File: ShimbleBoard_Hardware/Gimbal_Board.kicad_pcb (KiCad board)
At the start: 2 copper layers, 85 parts, among them Q1 Q_NMOS_GDS, Q2 Q_NMOS_GDS, Q3 Q_NMOS_GDS, Q4 Q_NMOS_GDS, Q5 Q_NMOS_GDS, Q6 Q_NMOS_GDS, Q7 Q_NMOS_GDS, Q8 Q_NMOS_GDS, SW1 SW_Push, SW10 SW_SPDT, SW2 SW_Push, SW3 SW_Push, SW4 SW_Push, SW5 SW_Push, SW6 SW_Push, SW7 SW_Push, SW8 SW_Push, SW9 SW_Push, U1 TM4C129E_Launchpad, U2 OKI, U3 OKI

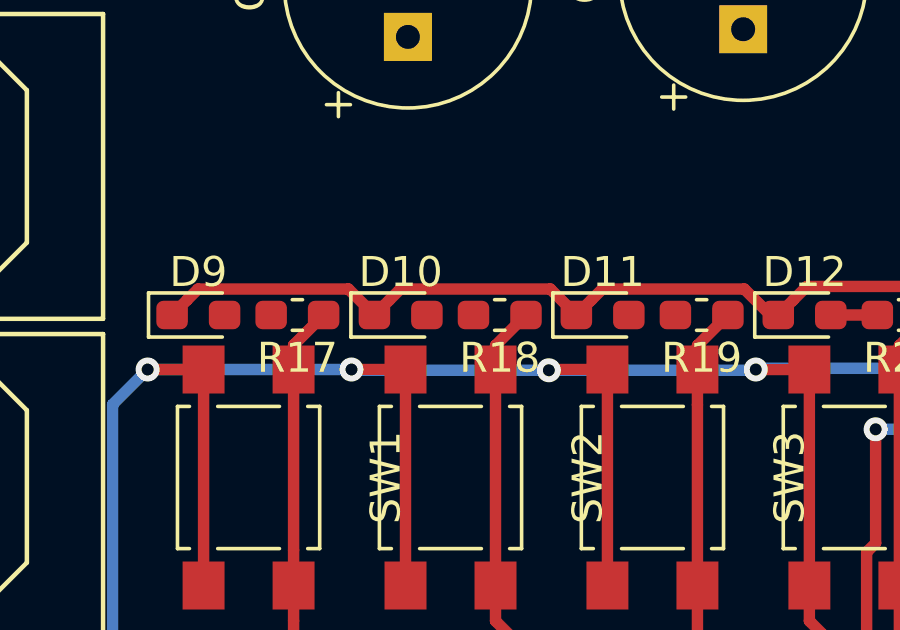
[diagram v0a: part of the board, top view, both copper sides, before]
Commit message: All Connected I Believe
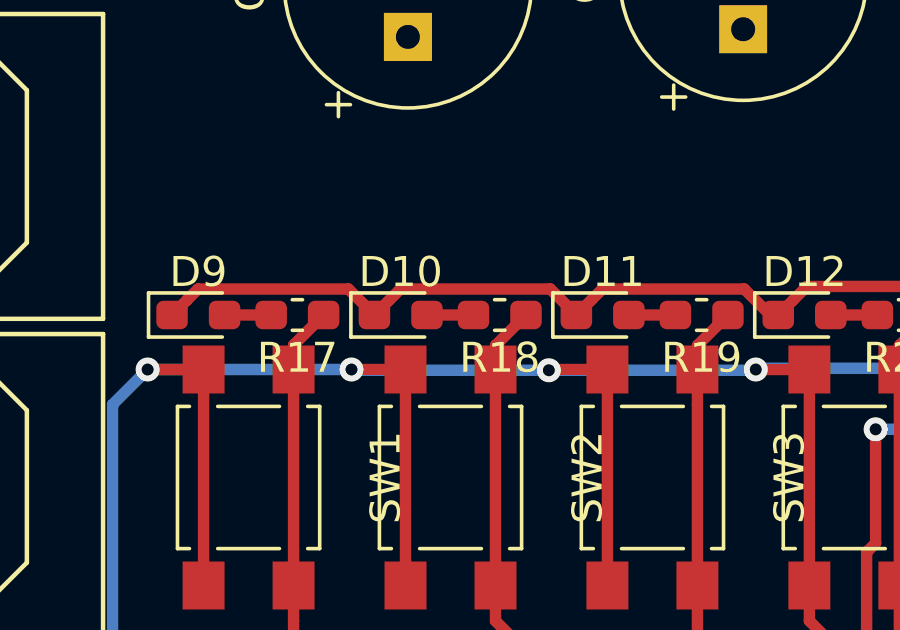
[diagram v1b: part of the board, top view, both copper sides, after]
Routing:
- net Net-(D9-Pad2): track 0.00 -> 1.55 mm
- net Net-(D11-Pad2): track 0.00 -> 1.55 mm
- net Net-(D10-Pad2): track 0.00 -> 1.55 mm
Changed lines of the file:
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@@
     (thickness 1.6)
     (drawings 1)
-    (tracks 401)
+    (tracks 404)
     (zones 0)
     (modules 85)
@@
   (segment (start 162.052 66.576) (end 162.842 65.786) (width 0.381) (layer F.Cu) (net 29))
   (segment (start 162.052 67.31) (end 162.052 66.576) (width 0.381) (layer F.Cu) (net 29))
+  (segment (start 113.27 90.551) (end 114.822 90.551) (width 0.381) (layer F.Cu) (net 30))
+  (segment (start 121.567 90.551) (end 120.015 90.551) (width 0.381) (layer F.Cu) (net 31))
+  (segment (start 128.298 90.551) (end 126.746 90.551) (width 0.381) (layer F.Cu) (net 85))
   (segment (start 135.029 90.551) (end 133.477 90.551) (width 0.381) (layer F.Cu) (net 86))
   (segment (start 140.208 90.551) (end 141.76 90.551) (width 0.381) (layer F.Cu) (net 87))
